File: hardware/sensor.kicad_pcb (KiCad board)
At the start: 2 copper layers, 55 parts, among them P1 CONN_01X05, SW1 Reset, T1 BUK9Y22, U1 LMR16006, U2 CD74HC4046, U3 CD74HC4046, U4 Atmel_SAM_D09, U5 OPA376AIDCK, X1 UART, X2 60V

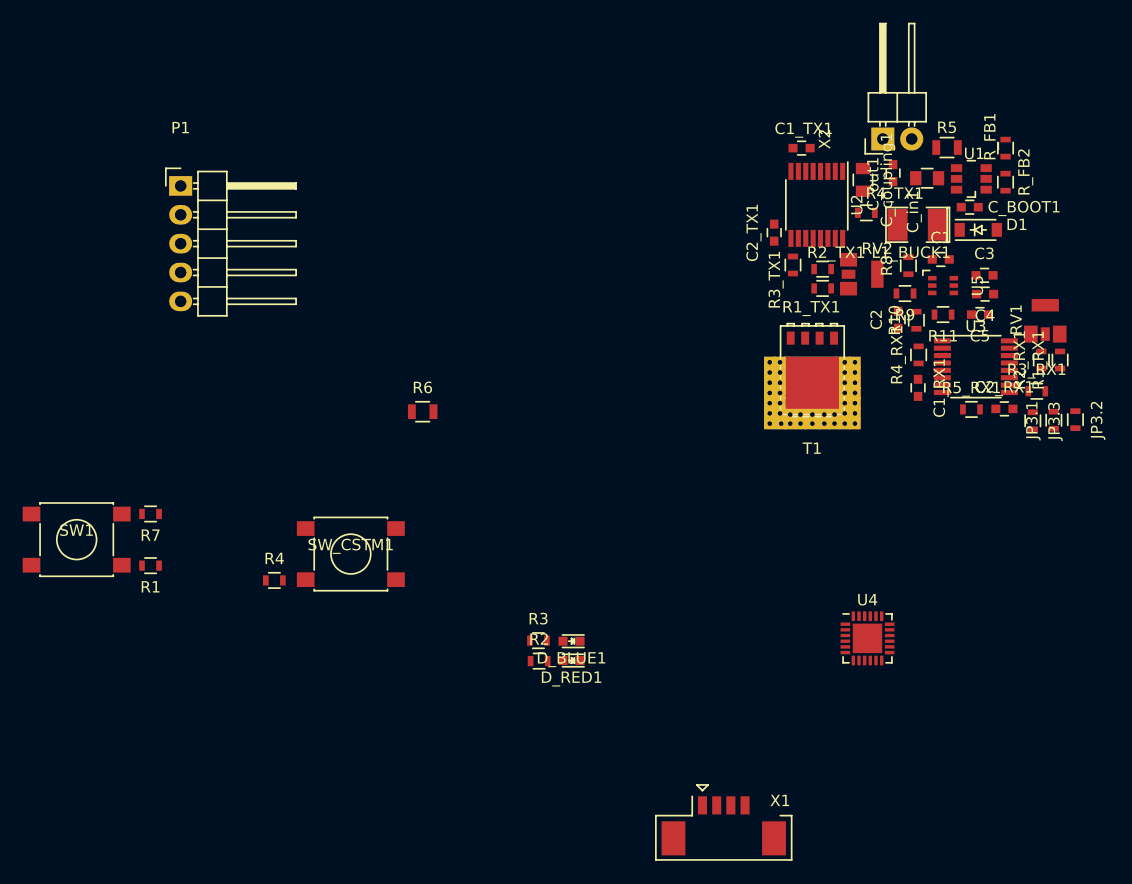
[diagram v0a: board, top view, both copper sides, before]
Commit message: Finished placing for now
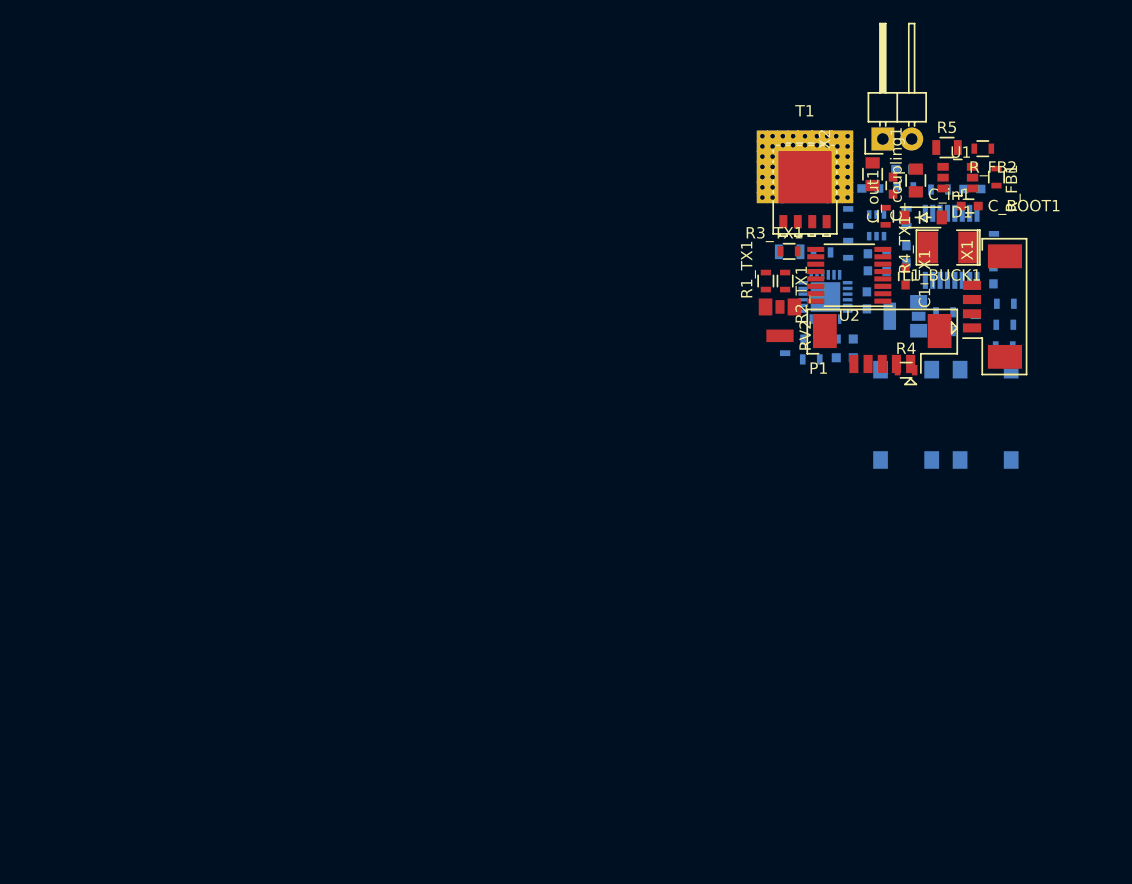
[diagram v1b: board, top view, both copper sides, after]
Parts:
- C1, C1_RX1, C2, C2_RX1, C2_TX1, C3, C4, C5, D_BLUE1, D_RED1, JP3.1, JP3.2, JP3.3, R10, R11, R1_RX1, R2, R2_RX1, R3, R3_RX1, R4_RX1, R5_RX1, R6, R7, R8, R9, RV1, SW1, SW_CSTM1, U3, U4, U5: moved to B.Cu
- P1: footprint Pin_Headers:Pin_Header_Angled_1x05 -> Connectors_Molex:Connector_Molex_PicoBlade_53261-0571
- R1: value R_Small -> 10k; moved to B.Cu
- moved SW1 80.8 mm to (168.9, 100.8), turned to 90 degrees
- moved R7 63.4 mm to (154.5, 86.5), turned to 0 degrees
- moved P1 63.1 mm to (159.8, 93.4), turned to 180 degrees
- moved R1 59.1 mm to (151.2, 94.6), turned to 90 degrees
- moved R4 58.6 mm to (161.9, 96.8)
- moved X1 52.9 mm to (170.6, 91.2), turned to 90 degrees
- moved SW_CSTM1 50.4 mm to (161.9, 100.8), turned to 270 degrees
- moved D_RED1 35.9 mm to (156.5, 95.8)
- moved D_BLUE1 35.9 mm to (156.5, 94.1)
- moved R3 35.8 mm to (153.6, 94.2)
- moved R2 35.8 mm to (153.6, 95.9)
- moved R6 35.2 mm to (151.7, 86.4)
- moved U4 30.3 mm to (154.8, 90.4), turned to 270 degrees
- moved C1_RX1 18.1 mm to (167.7, 80.9), turned to 0 degrees
- moved T1 15.9 mm to (153.0, 81.0), turned to 0 degrees
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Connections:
- R5_RX1 pad 2: /RX2_out -> /RX1_out
- U3 pad 10: /RX2_out -> /RX1_out
- U4 pad 22: /RX_in -> /RX1_out
- U4 pad 25: (no net) -> GND
